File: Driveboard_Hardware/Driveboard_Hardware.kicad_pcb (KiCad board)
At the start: 2 copper layers, 61 x 92.3 mm, 12 parts, among them U1 TM4C129E_Launchpad, U2 MAX_3232, U3 OKI

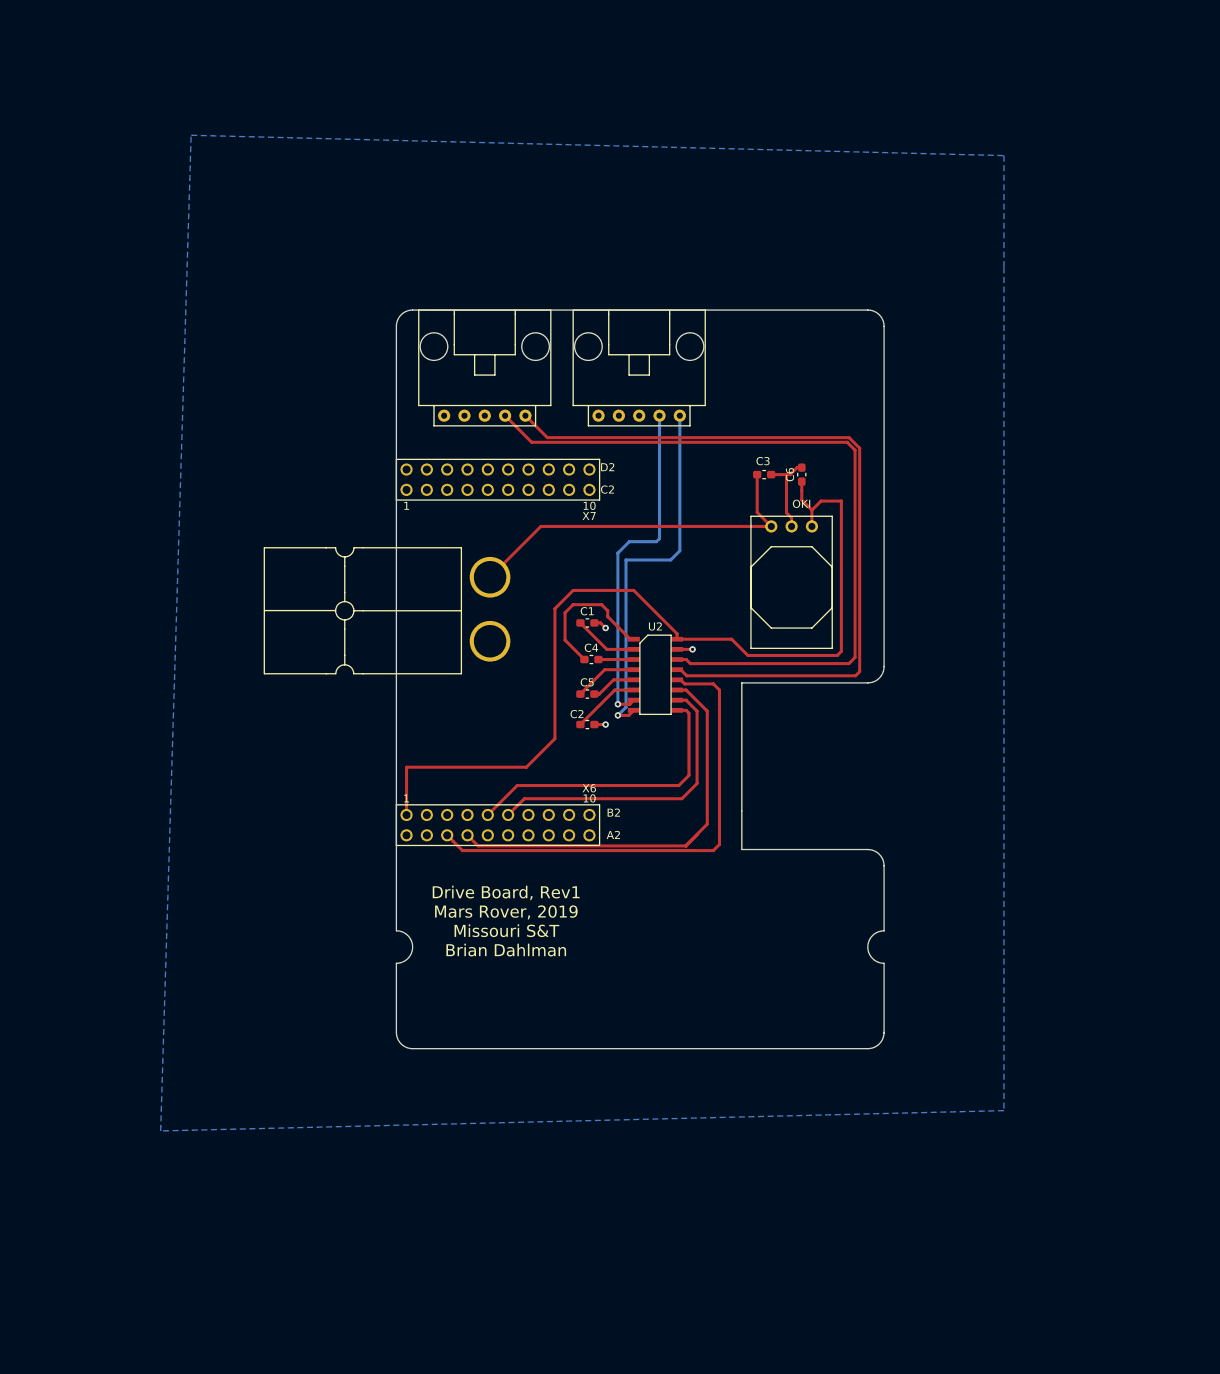
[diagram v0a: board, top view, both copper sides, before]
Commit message: Created Gerbs
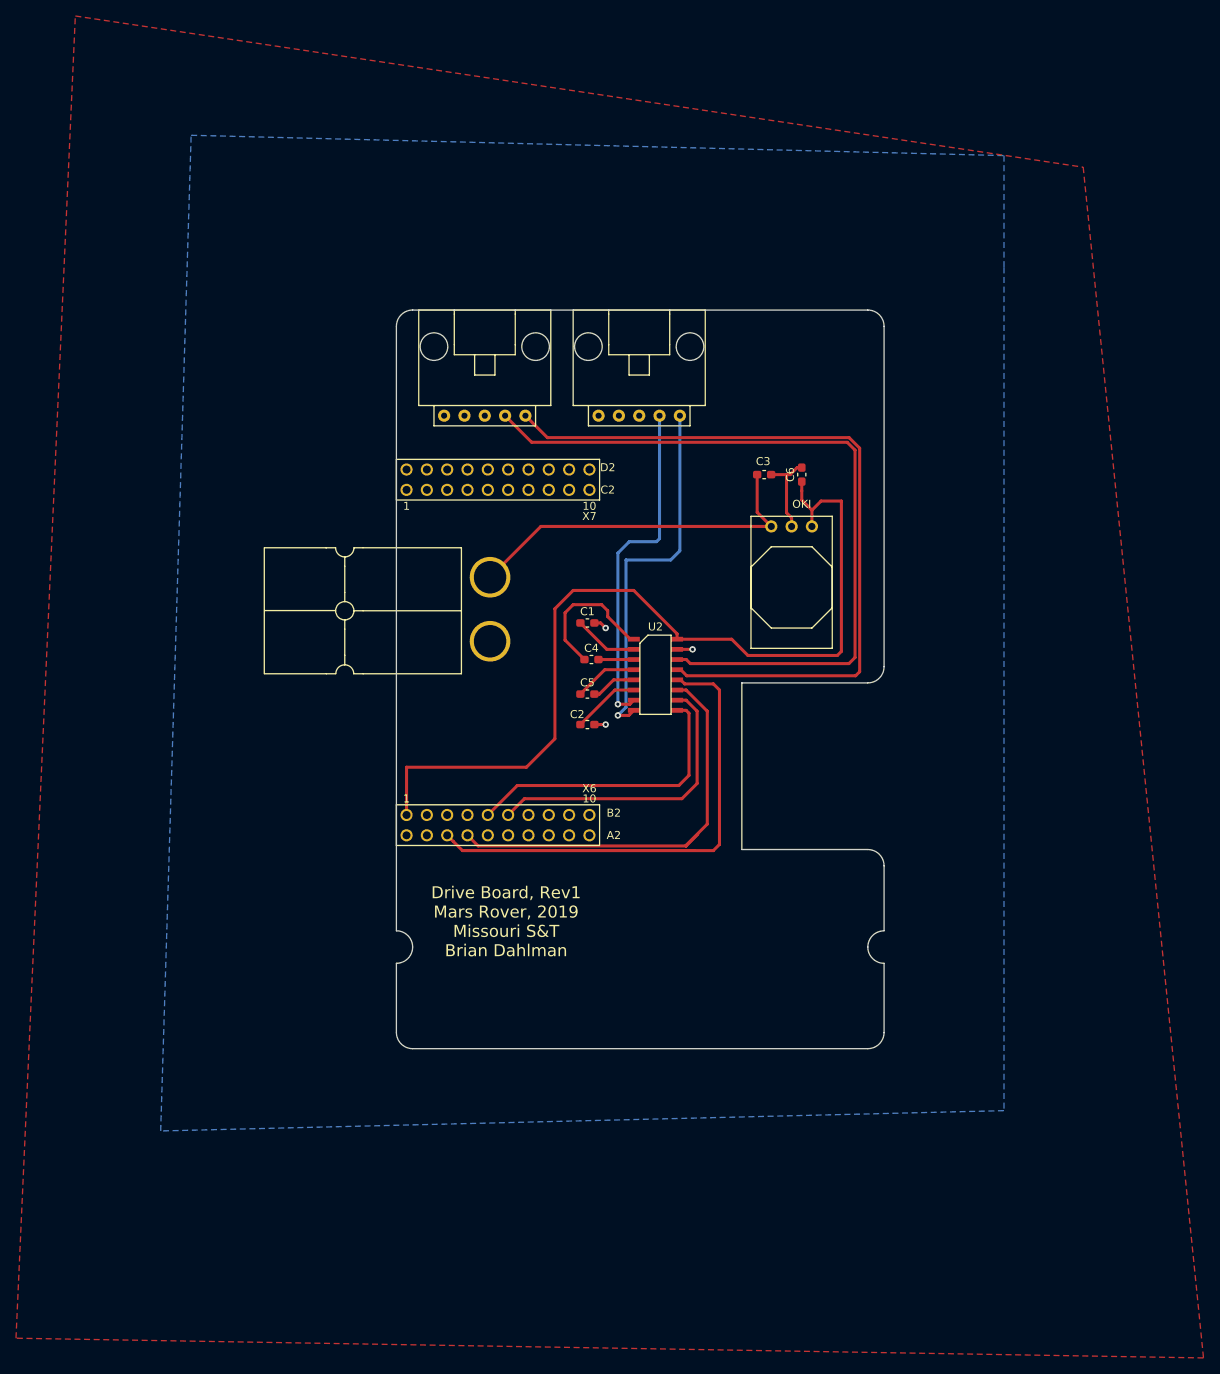
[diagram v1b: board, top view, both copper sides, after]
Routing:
- added copper zone on F.Cu, net GND
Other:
- outline, holes or cut-outs redrawn
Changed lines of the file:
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@@
   (general
     (thickness 1.6)
-    (drawings 20)
+    (drawings 21)
     (tracks 126)
     (zones 0)
@@
       (drillshape 0)
       (scaleselection 1)
-      (outputdirectory "../gerbs/"))
+      (outputdirectory "gerbs/"))
   )
   (net 0 "")
@@
       (net 9 +5V))
   )
+  (gr_line (start 74.676 52.324) (end 131.572 52.324) (layer Edge.Cuts) (width 0.15))
+  (gr_line (start 72.644 129.921) (end 72.644 54.356) (layer Edge.Cuts) (width 0.15))
+  (gr_line (start 72.644 142.621) (end 72.644 133.985) (layer Edge.Cuts) (width 0.15))
+  (gr_line (start 131.572 144.653) (end 74.676 144.653) (layer Edge.Cuts) (width 0.15))
+  (gr_line (start 133.604 142.621) (end 133.604 133.985) (layer Edge.Cuts) (width 0.15))
+  (gr_line (start 115.824 119.761) (end 131.572 119.761) (layer Edge.Cuts) (width 0.15))
+  (gr_line (start 115.824 98.933) (end 115.824 119.761) (layer Edge.Cuts) (width 0.15))
+  (gr_line (start 131.572 98.933) (end 115.824 98.933) (layer Edge.Cuts) (width 0.15))
+  (gr_line (start 133.604 54.356) (end 133.604 96.901) (layer Edge.Cuts) (width 0.15))
+  (gr_arc (start 131.572 54.356) (end 133.604 54.356) (angle -90) (layer Edge.Cuts) (width 0.15))
+  (gr_arc (start 74.676 54.356) (end 74.676 52.324) (angle -90) (layer Edge.Cuts) (width 0.15))
+  (gr_arc (start 131.572 96.901) (end 131.572 98.933) (angle -90) (layer Edge.Cuts) (width 0.15))
+  (gr_arc (start 72.644 131.953) (end 74.676 131.953) (angle -90) (layer Edge.Cuts) (width 0.15))
+  (gr_arc (start 72.644 131.953) (end 72.644 133.985) (angle -90) (layer Edge.Cuts) (width 0.15))
+  (gr_arc (start 74.676 142.621) (end 72.644 142.621) (angle -90) (layer Edge.Cuts) (width 0.15))
+  (gr_arc (start 131.572 142.621) (end 131.572 144.653) (angle -90) (layer Edge.Cuts) (width 0.15))
+  (gr_arc (start 133.604 131.953) (end 131.572 131.953) (angle -90) (layer Edge.Cuts) (width 0.15))
+  (gr_arc (start 133.604 131.953) (end 133.604 129.921) (angle -90) (layer Edge.Cuts) (width 0.15))
+  (gr_arc (start 131.572 121.793) (end 133.604 121.793) (angle -90) (layer Edge.Cuts) (width 0.15))
+  (gr_line (start 133.604 129.921) (end 133.604 121.793) (layer Edge.Cuts) (width 0.15))
   (gr_text "Drive Board, Rev1\nMars Rover, 2019\nMissouri S&T\nBrian Dahlman" (at 86.36 128.778) (layer F.SilkS)
     (effects (font (size 1.5 1.5) (thickness 0.3)))
   )
-  (gr_line (start 133.604 54.356) (end 133.604 96.901) (layer Edge.Cuts) (width 0.15))
-  (gr_line (start 74.676 52.324) (end 131.572 52.324) (layer Edge.Cuts) (width 0.15))
-  (gr_line (start 72.644 54.356) (end 72.644 129.921) (layer Edge.Cuts) (width 0.15))
-  (gr_arc (start 74.676 54.356) (end 74.676 52.324) (angle -90) (layer Edge.Cuts) (width 0.15))
-  (gr_arc (start 131.572 54.356) (end 133.604 54.356) (angle -90) (layer Edge.Cuts) (width 0.15))
-  (gr_line (start 131.572 144.653) (end 74.676 144.653) (layer Edge.Cuts) (width 0.15))
-  (gr_line (start 133.604 133.985) (end 133.604 142.748) (layer Edge.Cuts) (width 0.15))
-  (gr_line (start 133.604 121.793) (end 133.604 129.921) (layer Edge.Cuts) (width 0.15))
-  (gr_line (start 115.824 119.761) (end 131.572 119.761) (layer Edge.Cuts) (width 0.15))
-  (gr_line (start 115.824 114.935) (end 115.824 119.761) (layer Edge.Cuts) (width 0.15))
-  (gr_line (start 115.824 98.933) (end 115.824 114.935) (layer Edge.Cuts) (width 0.15))
-  (gr_line (start 131.572 98.933) (end 115.824 98.933) (layer Edge.Cuts) (width 0.15))
-  (gr_line (start 72.644 142.621) (end 72.644 133.985) (layer Edge.Cuts) (width 0.15))
-  (gr_arc (start 74.676 142.621) (end 72.644 142.621) (angle -90) (layer Edge.Cuts) (width 0.15))
-  (gr_arc (start 131.572 121.793) (end 133.604 121.793) (angle -90) (layer Edge.Cuts) (width 0.15))
-  (gr_arc (start 131.572 96.901) (end 131.572 98.933) (angle -90) (layer Edge.Cuts) (width 0.15))
-  (gr_arc (start 72.644 131.953) (end 72.644 133.985) (angle -180) (layer Edge.Cuts) (width 0.15))
-  (gr_arc (start 131.572 142.621) (end 131.572 144.653) (angle -90) (layer Edge.Cuts) (width 0.15))
-  (gr_arc (start 133.604 131.953) (end 133.604 129.921) (angle -180) (layer Edge.Cuts) (width 0.15))
   (segment (start 98.947 94.742) (end 95.645 91.44) (width 0.381) (layer F.Cu) (net 1))
   (segment (start 102.329 94.742) (end 98.947 94.742) (width 0.381) (layer F.Cu) (net 1))
@@
       )
     )
+  )
+  (zone (net 2) (net_name GND) (layer F.Cu) (hatch edge 0.508)
+    (connect_pads (clearance 0.508))
+    (min_thickness 0.254)
+    (fill yes (arc_segments 16) (thermal_gap 0.508) (thermal_bridge_width 0.508))
+    (polygon
+      (pts
+        (xy 158.496 34.4678) (xy 173.5328 183.3118) (xy 25.0952 180.848) (xy 32.512 15.5702)
+      )
+    )
